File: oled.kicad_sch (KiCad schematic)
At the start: 4 parts, among them J6 I2C_HEADER

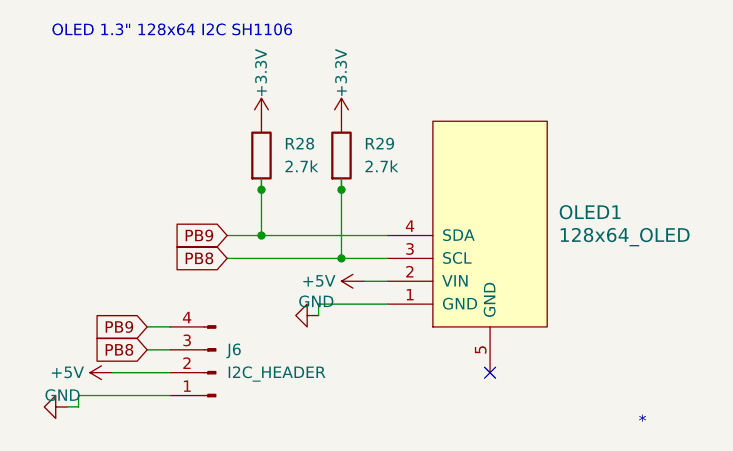
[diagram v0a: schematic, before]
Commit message: Solve all warnings
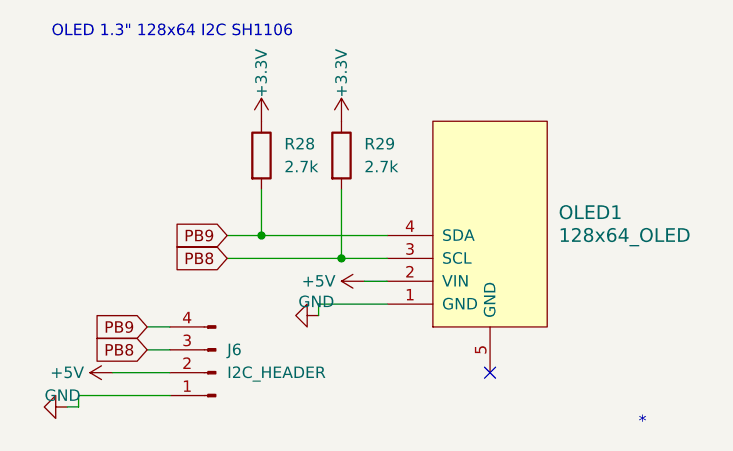
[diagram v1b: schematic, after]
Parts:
- OLED1: footprint Connector_PinHeader_2.54mm:2.42 OLED Simon Karl Custom -> ksoloti_shield_footprints:128x64OLED_1_3in; symbol ksoloti:display_i2c_oled -> ksoloti_shield_symbols:display_i2c_oled
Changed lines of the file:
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@@
 	)
 	(junction
-		(at 143.51 90.17)
+		(at 143.51 97.79)
 		(diameter 0)
 		(color 0 0 0 0)
@@
 		(color 0 0 0 0)
 	)
-	(junction
-		(at 143.51 97.79)
-		(diameter 0)
-		(color 0 0 0 0)
-	)
-	(junction
-		(at 134.62 90.17)
-		(diameter 0)
-		(color 0 0 0 0)
-	)
 	(no_connect
 		(at 160.02 110.49)
@@
 	(wire
 		(pts
+			(xy 134.62 95.25) (xy 148.59 95.25)
+		)
+		(stroke
+			(width 0)
+			(type default)
+		)
+	)
+	(wire
+		(pts
+			(xy 134.62 90.17) (xy 134.62 95.25)
+		)
+		(stroke
+			(width 0)
+			(type default)
+		)
+	)
+	(wire
+		(pts
+			(xy 114.3 114.3) (xy 113.03 114.3)
+		)
+		(stroke
+			(width 0)
+			(type default)
+		)
+	)
+	(wire
+		(pts
+			(xy 121.92 107.95) (xy 124.46 107.95)
+		)
+		(stroke
+			(width 0)
+			(type default)
+		)
+	)
+	(wire
+		(pts
+			(xy 140.97 102.87) (xy 148.59 102.87)
+		)
+		(stroke
+			(width 0)
+			(type default)
+		)
+	)
+	(wire
+		(pts
 			(xy 130.81 97.79) (xy 143.51 97.79)
 		)
@@
 	(wire
 		(pts
-			(xy 114.3 114.3) (xy 113.03 114.3)
+			(xy 118.11 110.49) (xy 124.46 110.49)
 		)
 		(stroke
@@
 	(wire
 		(pts
-			(xy 121.92 107.95) (xy 124.46 107.95)
-		)
-		(stroke
-			(width 0)
-			(type default)
-		)
-	)
-	(wire
-		(pts
-			(xy 143.51 88.9) (xy 143.51 90.17)
-		)
-		(stroke
-			(width 0)
-			(type default)
-		)
-	)
-	(wire
-		(pts
-			(xy 140.97 102.87) (xy 148.59 102.87)
-		)
-		(stroke
-			(width 0)
-			(type default)
-		)
-	)
-	(wire
-		(pts
-			(xy 134.62 90.17) (xy 134.62 95.25)
-		)
-		(stroke
-			(width 0)
-			(type default)
-		)
-	)
-	(wire
-		(pts
-			(xy 134.62 95.25) (xy 148.59 95.25)
+			(xy 140.97 102.87) (xy 140.97 104.14)
+		)
+		(stroke
+			(width 0)
+			(type default)
+		)
+	)
+	(wire
+		(pts
+			(xy 130.81 95.25) (xy 134.62 95.25)
 		)
 		(stroke
@@
 		(pts
 			(xy 143.51 97.79) (xy 148.59 97.79)
-		)
-		(stroke
-			(width 0)
-			(type default)
-		)
-	)
-	(wire
-		(pts
-			(xy 118.11 110.49) (xy 124.46 110.49)
-		)
-		(stroke
-			(width 0)
-			(type default)
-		)
-	)
-	(wire
-		(pts
-			(xy 134.62 88.9) (xy 134.62 90.17)
-		)
-		(stroke
-			(width 0)
-			(type default)
-		)
-	)
-	(wire
-		(pts
-			(xy 140.97 102.87) (xy 140.97 104.14)
-		)
-		(stroke
-			(width 0)
-			(type default)
-		)
-	)
-	(wire
-		(pts
-			(xy 130.81 95.25) (xy 134.62 95.25)
 		)
 		(stroke
@@
 	)
 	(symbol
-		(lib_id "ksoloti:display_i2c_oled")
+		(lib_id "ksoloti_shield_symbols:display_i2c_oled")
 		(at 148.59 102.87 0)
 		(unit 1)
@@
 			)
 		)
-		(property "Footprint" "Connector_PinHeader_2.54mm:2.42 OLED Simon Karl Custom"
+		(property "Footprint" "ksoloti_shield_footprints:128x64OLED_1_3in"
 			(at 158.75 106.68 0)
 			(effects
